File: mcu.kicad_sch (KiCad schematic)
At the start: 1 part, among them U1 MIMXRT1052CVJ5B

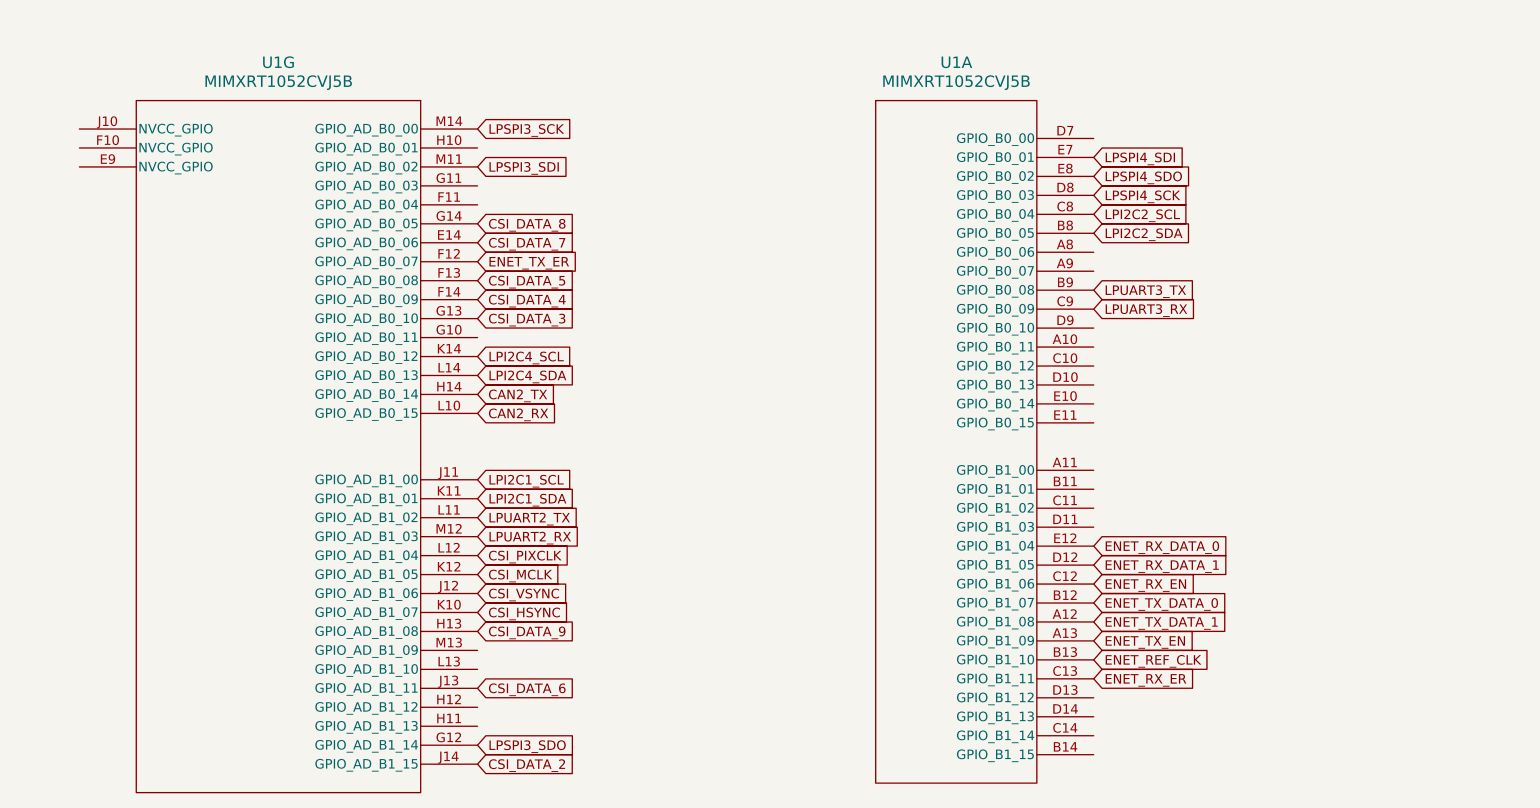
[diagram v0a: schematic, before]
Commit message: finished v1
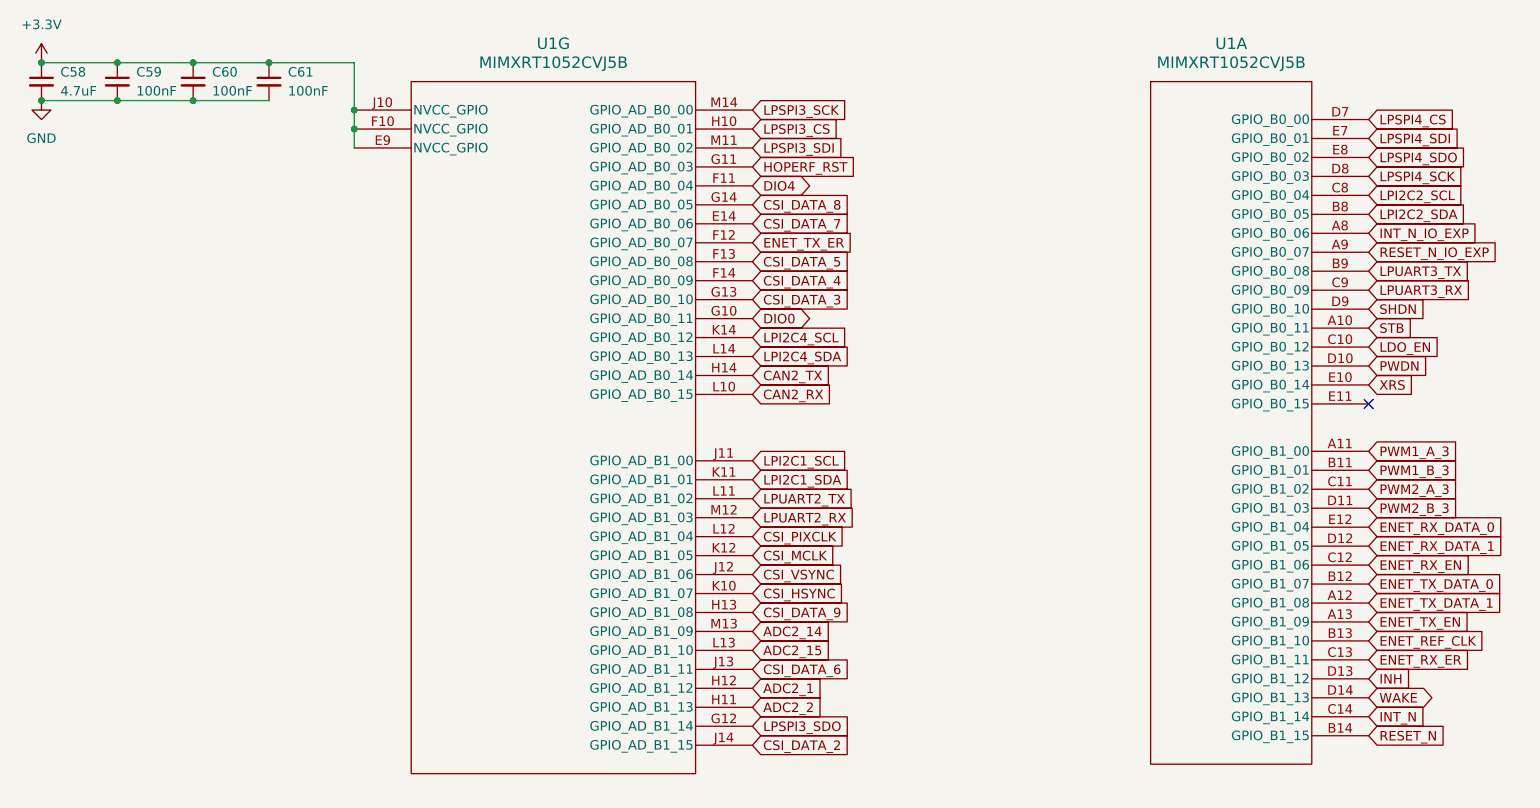
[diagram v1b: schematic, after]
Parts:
- added C58: 4.7uF, symbol Device:C_Small
- added C59, C60, C61: 100nF, symbol Device:C_Small
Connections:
- net +3.3V: now reaches U1.E9 (NVCC_GPIO)
- net +3.3V: now also U1.F10 (NVCC_GPIO), U1.J10 (NVCC_GPIO), C58.1, C59.1, C60.1, C61.1
- net DIO4: now reaches U1.F11 (GPIO_AD_B0_04)
- net DIO0: now reaches U1.G10 (GPIO_AD_B0_11)
- net HOPERF_RST: now reaches U1.G11 (GPIO_AD_B0_03)
- net LPSPI3_CS: now reaches U1.H10 (GPIO_AD_B0_01)
- net ADC2_2: now reaches U1.H11 (GPIO_AD_B1_13)
- net ADC2_1: now reaches U1.H12 (GPIO_AD_B1_12)
- net ADC2_15: now reaches U1.L13 (GPIO_AD_B1_10)
- net ADC2_14: now reaches U1.M13 (GPIO_AD_B1_09)
- net STB: now reaches U1.A10 (GPIO_B0_11)
- net PWM1_A_3: now reaches U1.A11 (GPIO_B1_00)
- net INT_N_IO_EXP: now reaches U1.A8 (GPIO_B0_06)
- net RESET_N_IO_EXP: now reaches U1.A9 (GPIO_B0_07)
- net PWM1_B_3: now reaches U1.B11 (GPIO_B1_01)
- net RESET_N: now reaches U1.B14 (GPIO_B1_15)
- net LDO_EN: now reaches U1.C10 (GPIO_B0_12)
- net PWM2_A_3: now reaches U1.C11 (GPIO_B1_02)
- net INT_N: now reaches U1.C14 (GPIO_B1_14)
- net PWDN: now reaches U1.D10 (GPIO_B0_13)
- net PWM2_B_3: now reaches U1.D11 (GPIO_B1_03)
- net INH: now reaches U1.D13 (GPIO_B1_12)
- net WAKE: now reaches U1.D14 (GPIO_B1_13)
- net LPSPI4_CS: now reaches U1.D7 (GPIO_B0_00)
- net SHDN: now reaches U1.D9 (GPIO_B0_10)
- net XRS: now reaches U1.E10 (GPIO_B0_14)
- new net GND: C58.2, C59.2, C60.2, C61.2
- no-connect marks 0 -> 1
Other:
- company: (none) -> Northeastern University
- title: (none) -> RT1050 DevBoard for Project Horizon
- moved on the sheet: U1A, U1G
